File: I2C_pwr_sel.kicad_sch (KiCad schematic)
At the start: 1 part, among them U408 TCA9535DBR

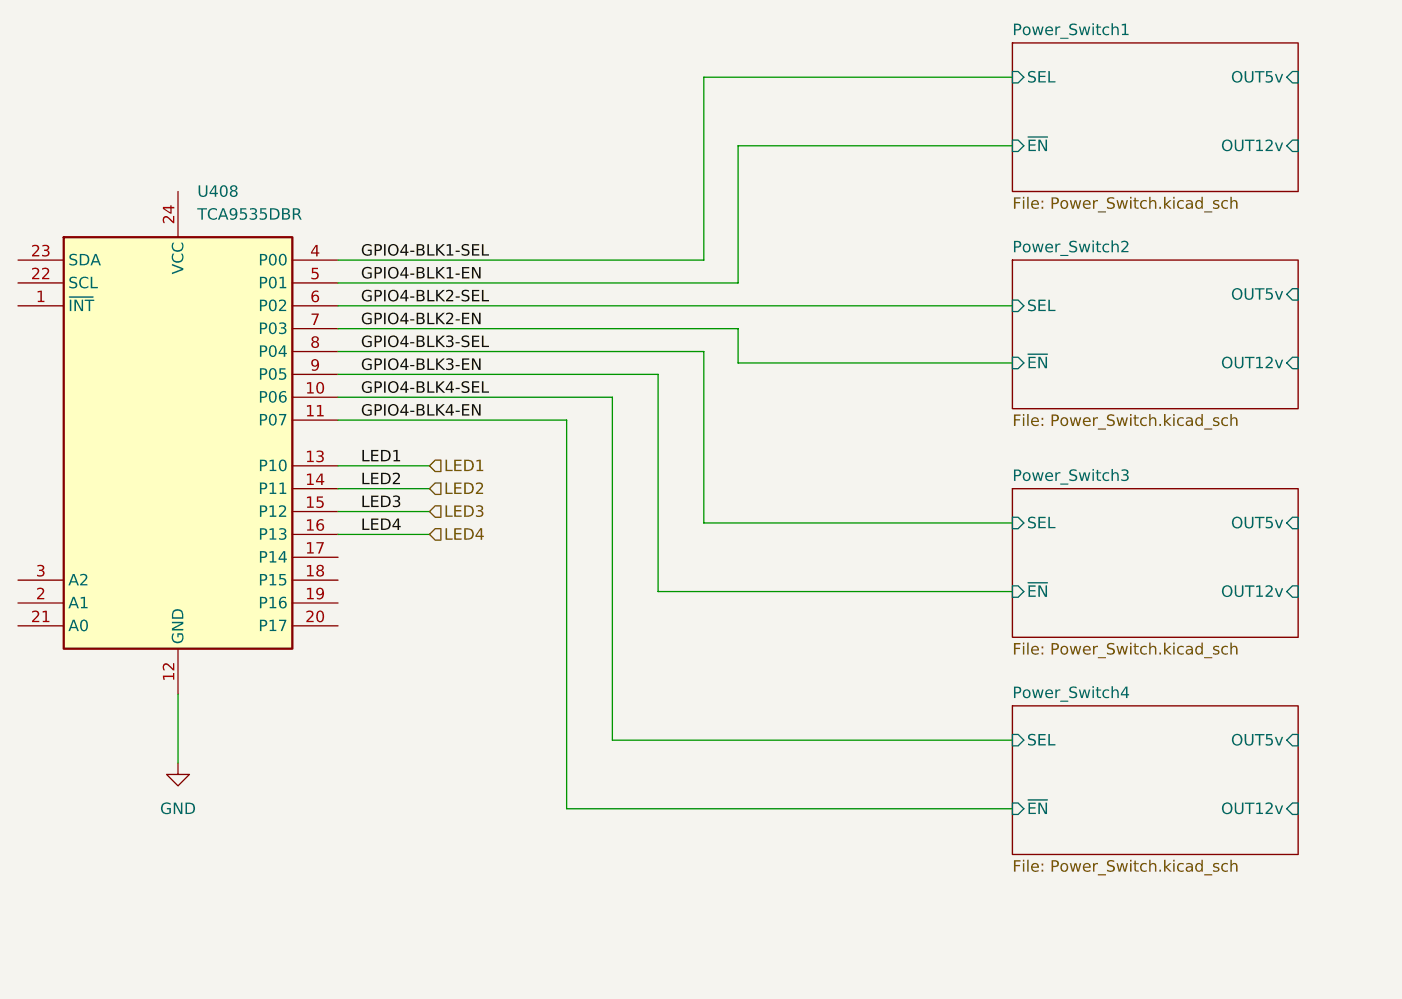
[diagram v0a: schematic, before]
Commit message: layout go brrr
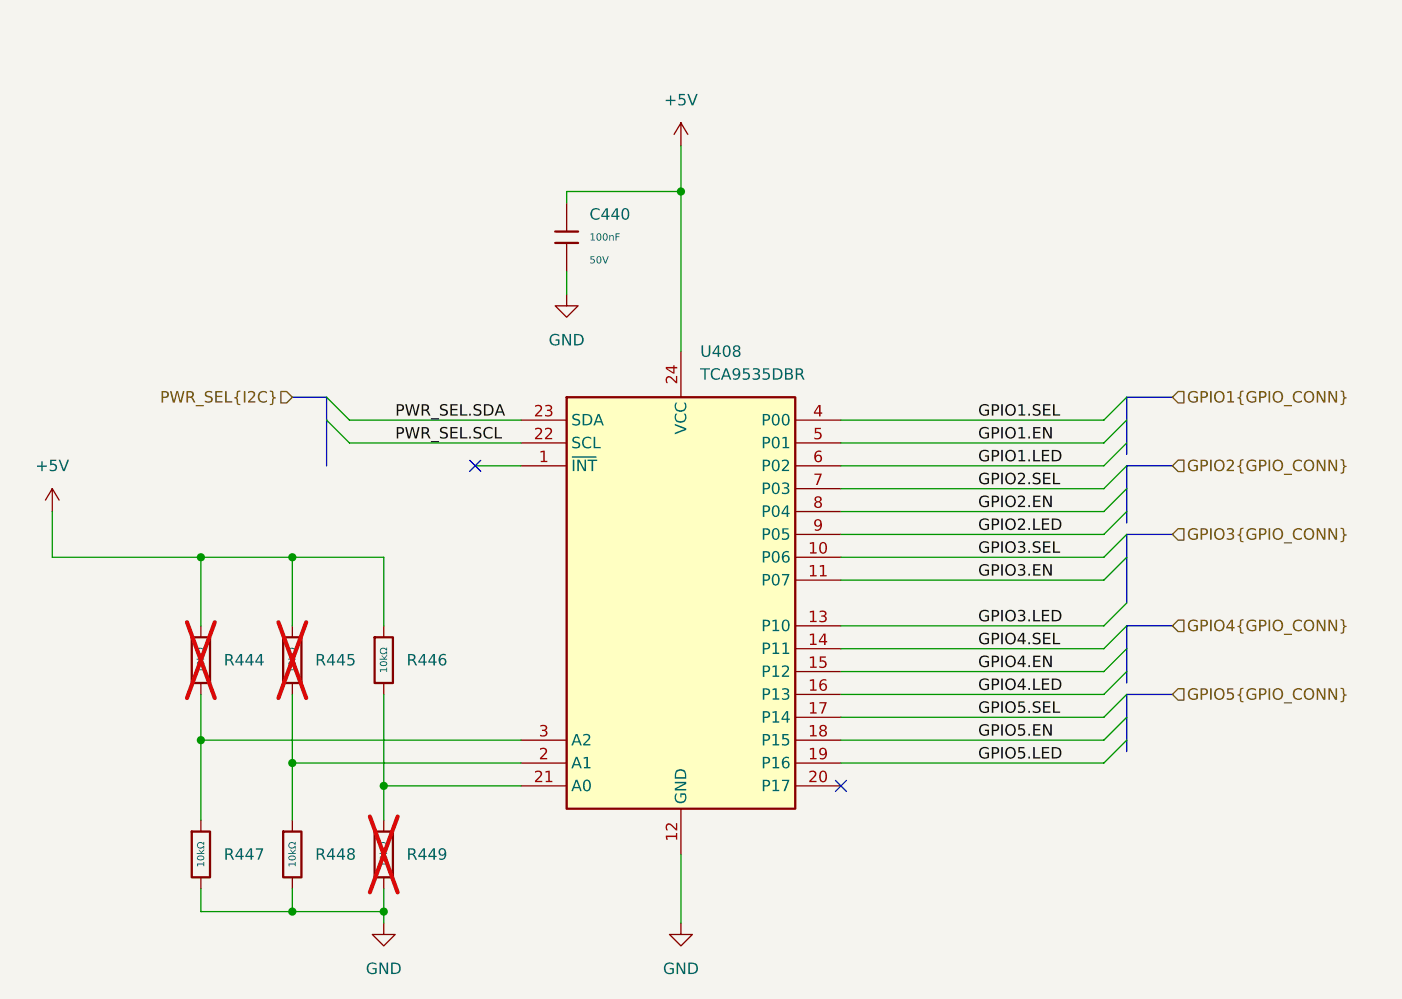
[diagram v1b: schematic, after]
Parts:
- added C440: 100nF, PCM_JLCPCB:C_0402, symbol PCM_JLCPCB-Capacitors:0402,100nF,(2)
- added R444, R445, R446, R447, R448, R449: 10kΩ, PCM_JLCPCB:R_0402, symbol PCM_JLCPCB-Resistors:0402,10kΩ
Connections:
- net GND: now also C440.2, R447.2, R448.2, R449.2
- net GPIO5.SEL: now reaches U408.17 (P14)
- net GPIO5.EN: now reaches U408.18 (P15)
- net GPIO5.LED: now reaches U408.19 (P16)
- net at U408.2 (A1): now also R445.2, R448.1
- net at U408.21 (A0): now also R446.2, R449.1
- net PWR_SEL.SCL: now reaches U408.22 (SCL)
- net PWR_SEL.SDA: now reaches U408.23 (SDA)
- net +5V: now reaches U408.24 (VCC)
- net +5V: now also C440.1, R444.1, R445.1, R446.1
- net at U408.3 (A2): now also R444.2, R447.1
- net GPIO4-BLK1-EN renamed GPIO1.EN
- net GPIO4-BLK1-SEL renamed GPIO1.SEL
- net GPIO4-BLK2-EN renamed GPIO2.SEL
- net GPIO4-BLK2-SEL renamed GPIO1.LED
- net GPIO4-BLK3-EN renamed GPIO2.LED
- net GPIO4-BLK3-SEL renamed GPIO2.EN
- net GPIO4-BLK4-EN renamed GPIO3.EN
- net GPIO4-BLK4-SEL renamed GPIO3.SEL
- net LED1 renamed GPIO3.LED
- net LED2 renamed GPIO4.SEL
- net LED3 renamed GPIO4.EN
- net LED4 renamed GPIO4.LED
- no-connect marks 0 -> 2
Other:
- removed sheet Power_Switch1
- removed sheet Power_Switch2
- removed sheet Power_Switch3
- removed sheet Power_Switch4
- moved on the sheet: U408
